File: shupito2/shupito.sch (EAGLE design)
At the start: 81 parts, among them IC2 74LVC1T45, IC3 74LVC1T45, IC4 74LVC1T45, IC5 74LVC1T45, IC6 ATXMEGA32A4U-AU, IC7 TPS73033DBV, Q1 BC807W-1907646, Q10 1758094, Q11 PDTC123YU-1757992, Q2 NX2301P-1894738, Q3 BC807W-1907646, Q4 PDTC123YU-1757992, Q5 PDTC123YU-1757992, Q7 PDTC123YU-1757992, Q8 PDTC123YU-1757992, X2 USB-MICRO-B-BOTTOM

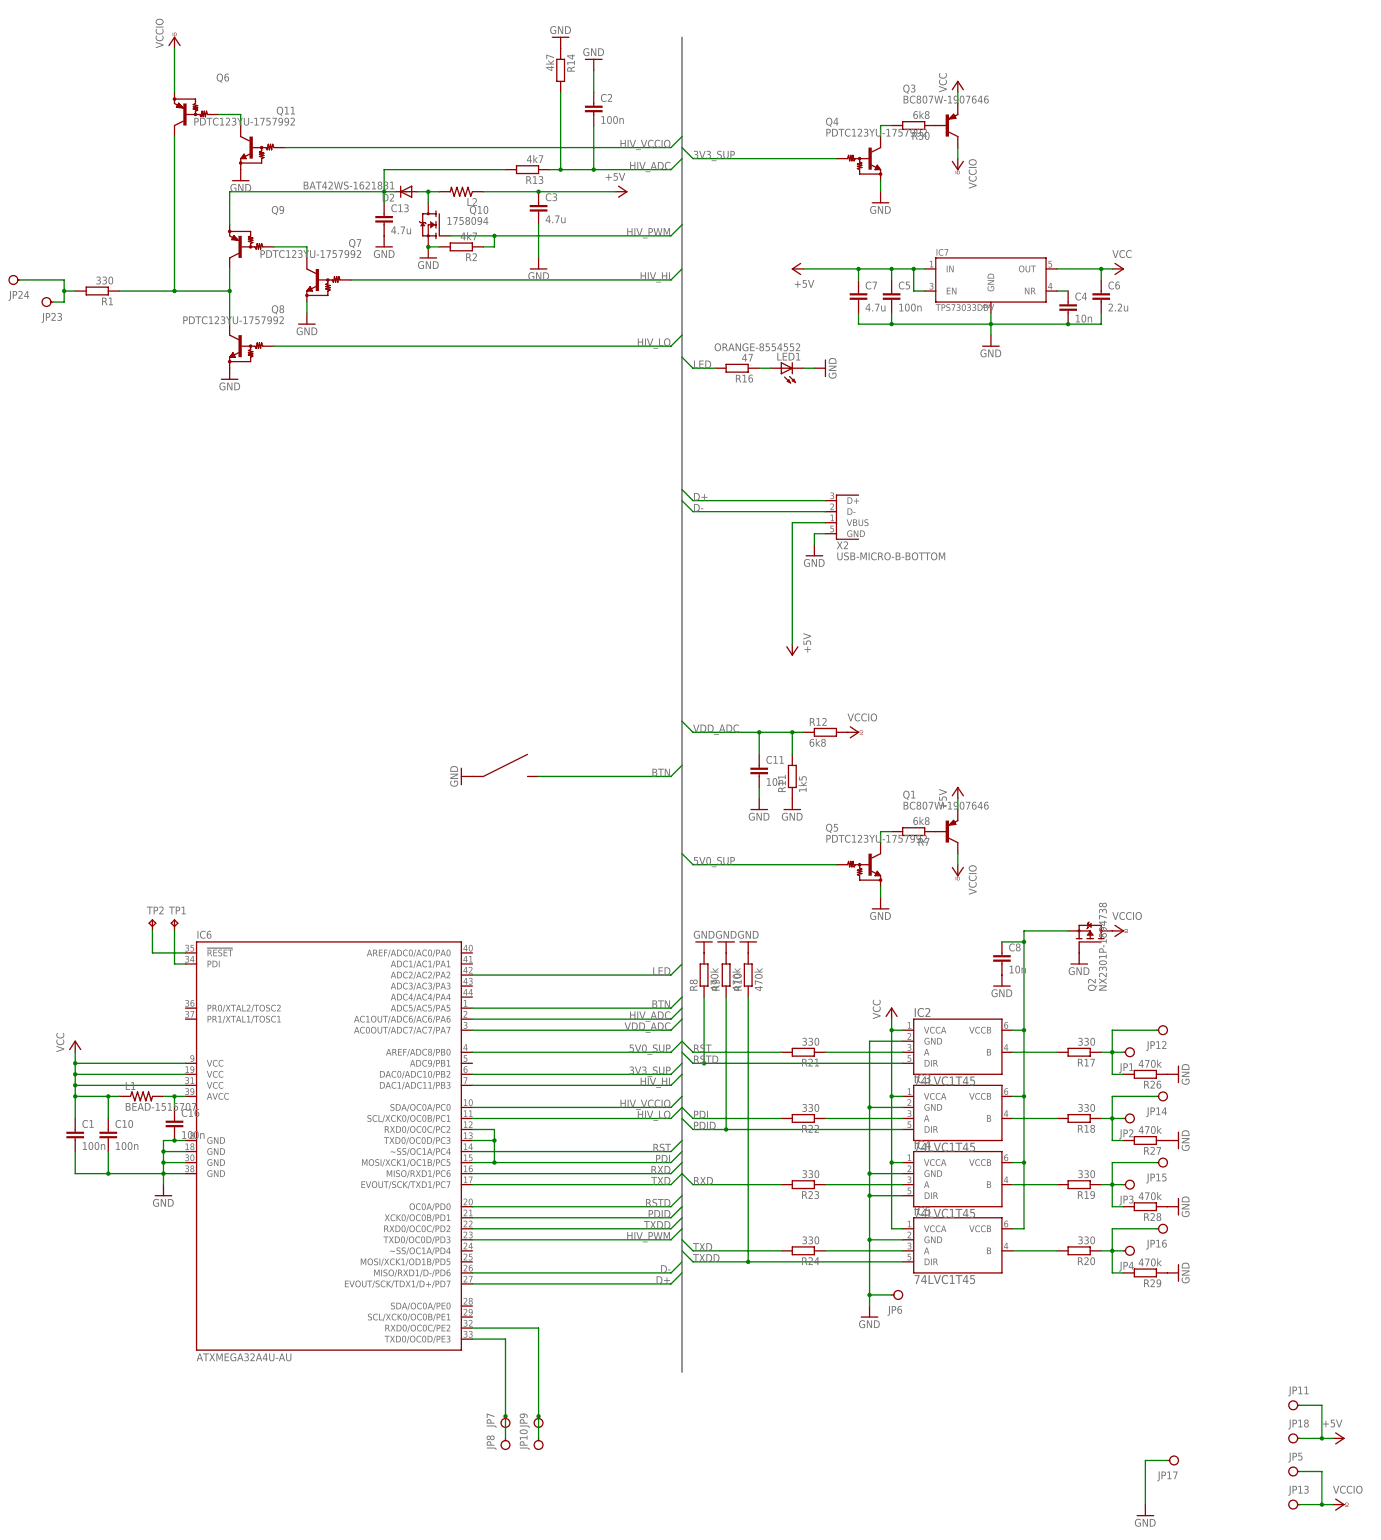
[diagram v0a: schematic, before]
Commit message: Routed.
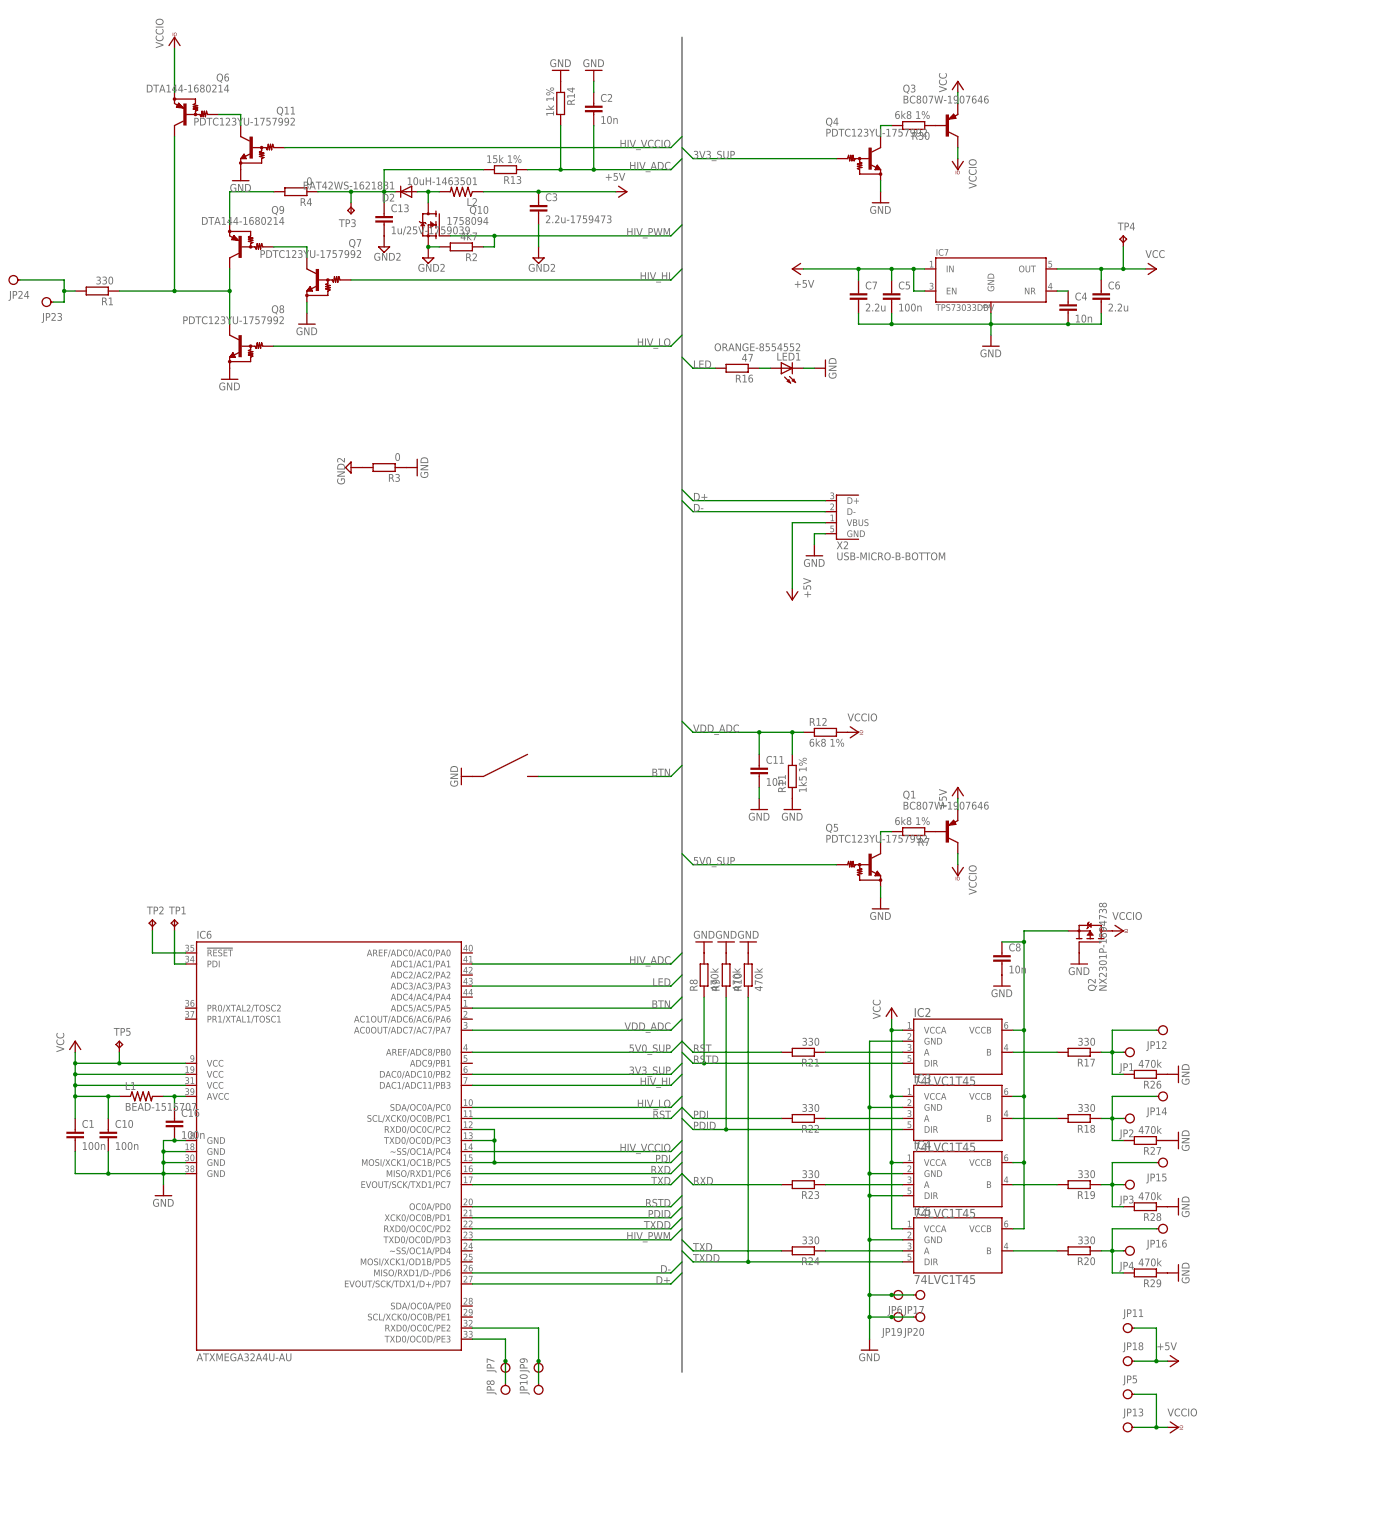
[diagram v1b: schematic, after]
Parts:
- added JP19, JP20: PINH1X01SMD, pinhead_smd:PINH1X01SMD
- added R3, R4: 0, rcl:R-EU_R1206
- added TP3, TP4, TP5: TPTP15SQ, testpad:TPTP15SQ
- C1, C11, C4, C5, C8: device rcl:C-EUC0603 -> rcl:C-EUC0603K
- C13: value 4.7u -> 1u/25V-1759039; device rcl:C-EUC0603 -> rcl:C-EUC0603K
- C2: value 100n -> 10n; device rcl:C-EUC0603 -> rcl:C-EUC0603K
- C3: value 4.7u -> 2.2u-1759473; device rcl:C-EUC1206 -> rcl:C-EUC0603K
- C6: device rcl:C-EUC1206 -> rcl:C-EUC0603K
- C7: value 4.7u -> 2.2u; device rcl:C-EUC1206 -> rcl:C-EUC0603K
- L2: value (none) -> 10uH-1463501; device rcl:R-US_R0603 -> rcl:R-US_R0805
- Q6, Q9: value (none) -> DTA144-1680214
- R11: value 1k5 -> 1k5 1%
- R12, R30, R7: value 6k8 -> 6k8 1%
- R13: value 4k7 -> 15k 1%
- R14: value 4k7 -> 1k 1%
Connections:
- new net GND2: C13.2, C3.2, Q10.S, R2.2, R3.2
- new net N$11: Q9.E, R4.2
- net GND: now also JP19.1, JP20.1, R3.1; no longer C13.2, C3.2, Q10.S, R2.2
- net HIV_ADC: now also IC6.ADC1/AC1/PA1; no longer IC6.AC1OUT/ADC6/AC6/PA6
- net HIV_LO: now also IC6.SDA/OC0A/PC0; no longer IC6.SCL/XCK0/OC0B/PC1
- net HIV_VCCIO: now also IC6.~SS/OC1A/PC4; no longer IC6.SDA/OC0A/PC0
- net LED: now also IC6.ADC3/AC3/PA3; no longer IC6.ADC2/AC2/PA2
- net N$22: now also R4.1, TP3.TP; no longer Q9.E
- net RST: now also IC6.SCL/XCK0/OC0B/PC1; no longer IC6.~SS/OC1A/PC4
- net VCC: now also TP4.TP, TP5.TP
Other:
- moved on the sheet: JP10, JP11, JP13, JP17, JP18, JP5, JP7, JP8, JP9, R13, R14

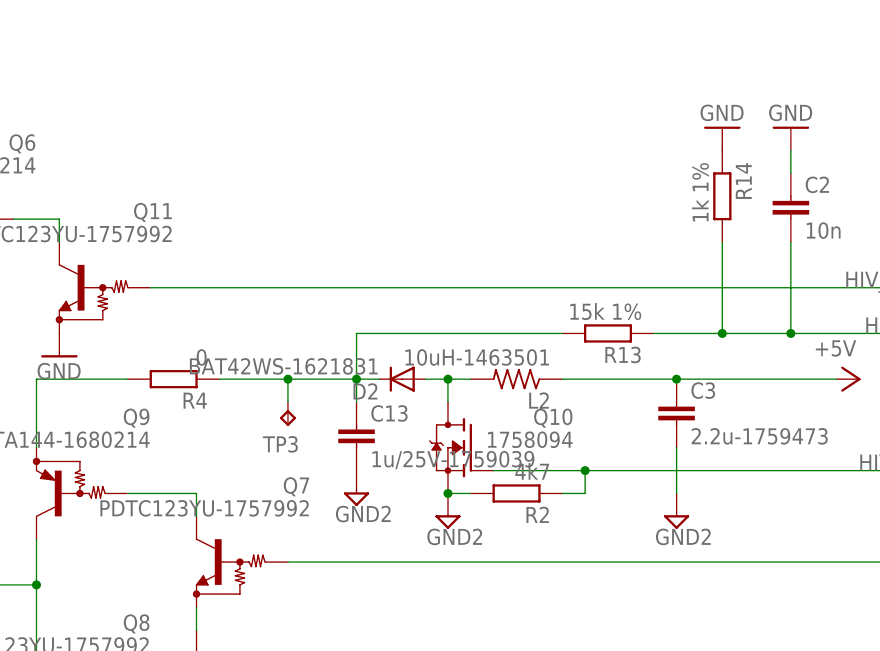
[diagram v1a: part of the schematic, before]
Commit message: Done.
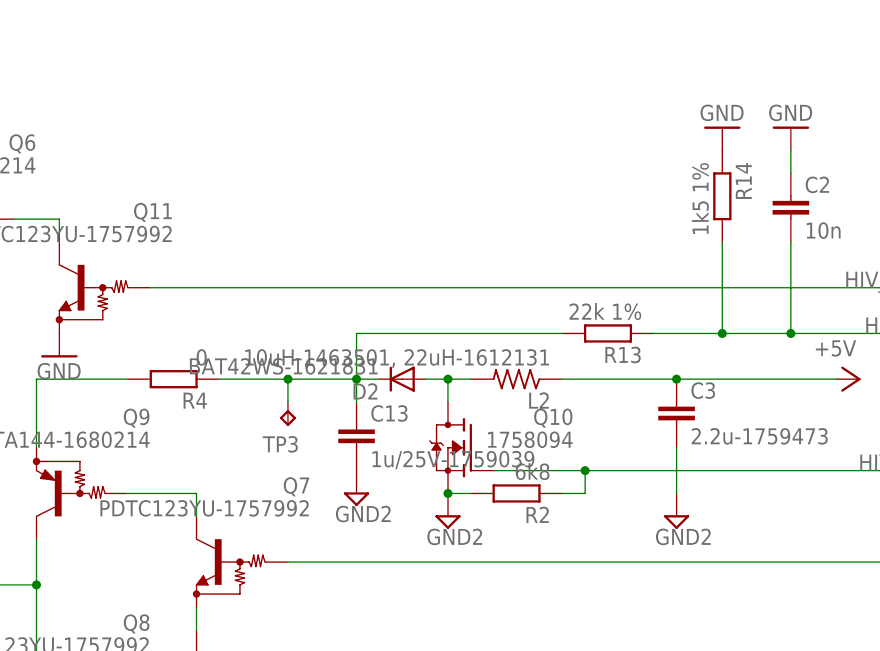
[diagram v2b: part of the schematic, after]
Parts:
- L2: value 10uH-1463501 -> 10uH-1463501, 22uH-1612131
- R13: value 15k 1% -> 22k 1%
- R14: value 1k 1% -> 1k5 1%
- R2: value 4k7 -> 6k8
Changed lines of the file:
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@@
 <part name="Q7" library="transistors" deviceset="NPN-BIAS" device="-SOT323-BEC" value="PDTC123YU-1757992"/>
 <part name="Q8" library="transistors" deviceset="NPN-BIAS" device="-SOT323-BEC" value="PDTC123YU-1757992"/>
-<part name="L2" library="rcl" deviceset="R-US_" device="R0805" value="10uH-1463501"/>
+<part name="L2" library="rcl" deviceset="R-US_" device="R0805" value="10uH-1463501, 22uH-1612131"/>
 <part name="C13" library="rcl" deviceset="C-EU" device="C0603K" value="1u/25V-1759039"/>
 <part name="D2" library="diode" deviceset="DIODE" device="-SOD323" value="BAT42WS-1621831"/>
 <part name="Q10" library="transistors" deviceset="N-MOSFET" device="-SOT323-GSD" value="1758094"/>
 <part name="R1" library="rcl" deviceset="R-EU_" device="R0603" value="330"/>
-<part name="R2" library="rcl" deviceset="R-EU_" device="R0603" value="4k7"/>
+<part name="R2" library="rcl" deviceset="R-EU_" device="R0603" value="6k8"/>
 <part name="Q9" library="transistors" deviceset="PNP-BIAS" device="-SOT323-BEC" value="DTA144-1680214"/>
-<part name="R13" library="rcl" deviceset="R-EU_" device="R0603" value="15k 1%"/>
-<part name="R14" library="rcl" deviceset="R-EU_" device="R0603" value="1k 1%"/>
+<part name="R13" library="rcl" deviceset="R-EU_" device="R0603" value="22k 1%"/>
+<part name="R14" library="rcl" deviceset="R-EU_" device="R0603" value="1k5 1%"/>
 <part name="GND23" library="supply1" deviceset="GND" device=""/>
 <part name="IC6" library="xmega" deviceset="ATXMEGA*A4U" device="-AU" technology="32"/>
